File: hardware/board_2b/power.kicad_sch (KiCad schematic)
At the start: 58 parts, among them J13 Conn_power, U1 Ti60F256, U18 TPS562211DRLR, U19 TPS562211DRLR, U20 TPS562211DRLR, U22 MAX77827AEFD, U26 MAX77827AEFD

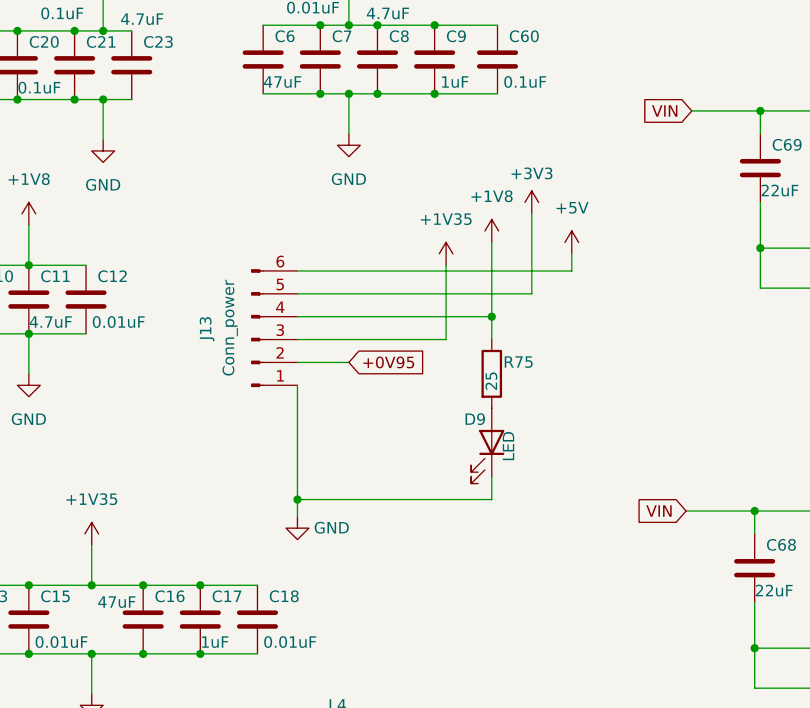
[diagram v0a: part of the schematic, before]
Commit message: Update hardware/board_2b
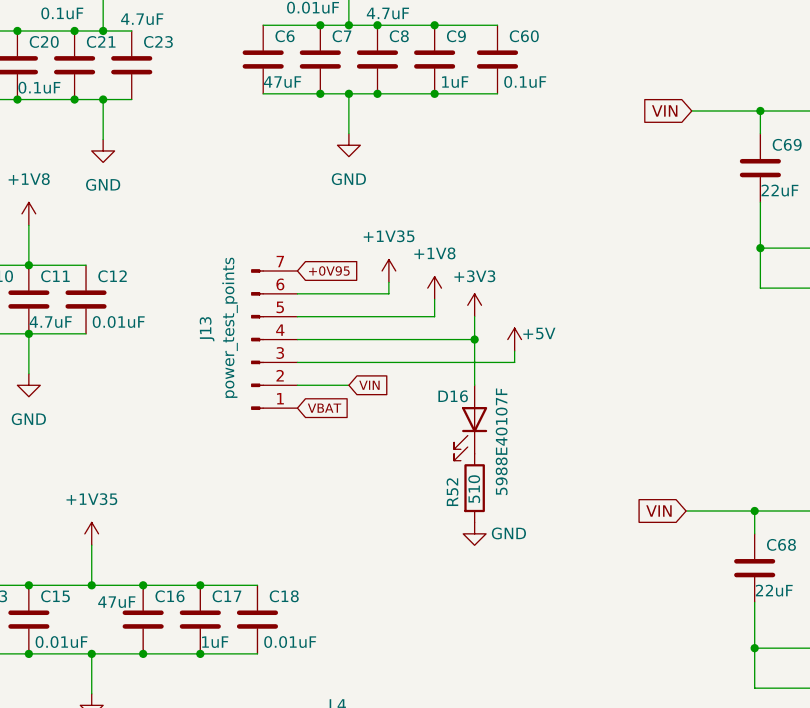
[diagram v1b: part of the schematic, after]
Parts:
- removed D9: LED, LED_SMD:LED_0603_1608Metric, symbol Device:LED
- removed R75: 25, Resistor_SMD:R_0603_1608Metric, symbol Device:R
- added D16: 5988E40107F, LED_SMD:LED_0603_1608Metric, symbol Device:LED
- added R52: 510, Resistor_SMD:R_0603_1608Metric, symbol Device:R
- J13: value Conn_power -> power_test_points; footprint Connector_PinHeader_2.54mm:PinHeader_2x03_P2.54mm_Vertical -> Connector_PinHeader_2.54mm:PinHeader_1x07_P2.54mm_Vertical; symbol Connector:Conn_01x06_Pin -> Connector:Conn_01x07_Pin
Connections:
- net +0V95: now also J13.7 (Pin_7); no longer J13.2 (Pin_2)
- net +1V35: now also J13.6 (Pin_6); no longer J13.3 (Pin_3)
- net +1V8: now also J13.5 (Pin_5); no longer J13.4 (Pin_4)
- net +3V3: now also J13.4 (Pin_4), D16.2 (A); no longer J13.5 (Pin_5)
- net +5V: now also J13.3 (Pin_3); no longer J13.6 (Pin_6)
- net GND: now also R52.2; no longer J13.1 (Pin_1)
- net VIN: now also J13.2 (Pin_2)
- new net: D16.1 (K), R52.1
- new net VBAT: J13.1 (Pin_1)
